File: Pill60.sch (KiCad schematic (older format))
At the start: 160 parts, among them J1 OLED, SW1 Rotary_Encoder_Switch, U1 ChinaBluePill

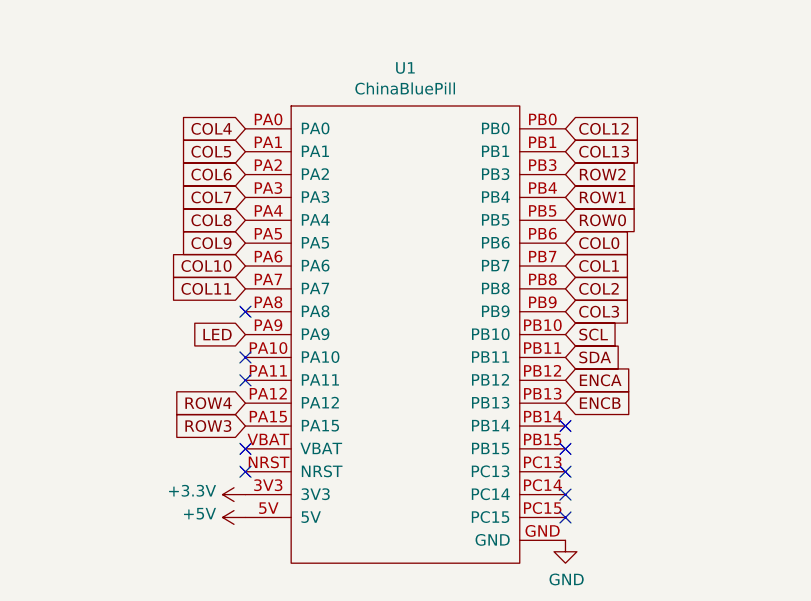
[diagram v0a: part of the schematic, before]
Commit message: Fix wires and make stuff better
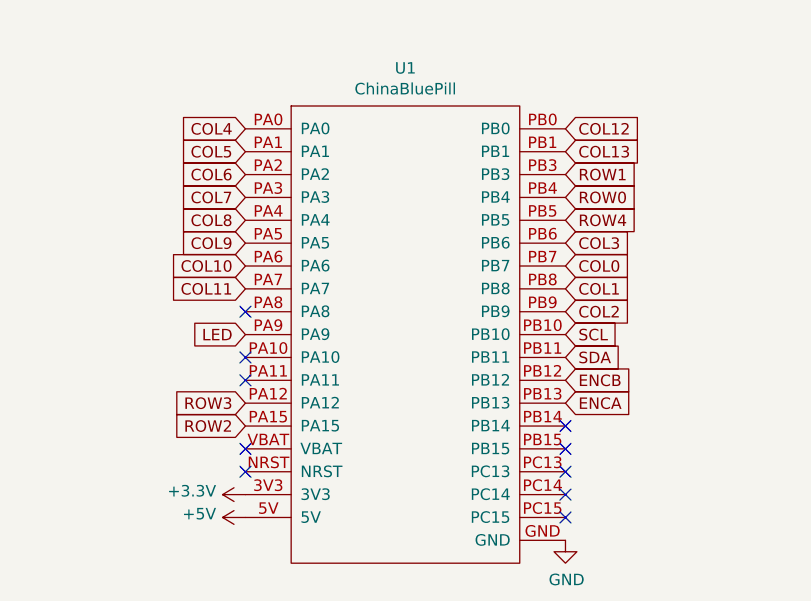
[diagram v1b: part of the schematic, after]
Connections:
- net COL0: now also U1.PB7; no longer U1.PB6
- net COL1: now also U1.PB8; no longer U1.PB7
- net COL2: now also U1.PB9; no longer U1.PB8
- net COL3: now also U1.PB6; no longer U1.PB9
- net ENCA: now also U1.PB13; no longer U1.PB12
- net ENCB: now also U1.PB12; no longer U1.PB13
- net ROW0: now also U1.PB4; no longer U1.PB5
- net ROW1: now also U1.PB3; no longer U1.PB4
- net ROW2: now also U1.PA15; no longer U1.PB3
- net ROW3: now also U1.PA12; no longer U1.PA15
- net ROW4: now also U1.PB5; no longer U1.PA12
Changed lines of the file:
@@
 Text GLabel 4950 1750 0    50   Input ~ 0
 ENCB
+Text GLabel 13100 3200 2    50   Input ~ 0
+ENCA
 Text GLabel 13100 3100 2    50   Input ~ 0
-ENCA
-Text GLabel 13100 3200 2    50   Input ~ 0
 ENCB
 $Comp
@@
 	0    -1   -1   0
 $EndComp
+Text GLabel 13100 2400 2    50   Input ~ 0
+ROW4
 Text GLabel 11700 3200 0    50   Input ~ 0
-ROW4
+ROW3
 Text GLabel 11700 3300 0    50   Input ~ 0
-ROW3
+ROW2
 Text GLabel 13100 2200 2    50   Input ~ 0
-ROW2
-Text GLabel 13100 2300 2    50   Input ~ 0
 ROW1
 $Comp
@@
 	1    0    0    -1
 $EndComp
+Text GLabel 13100 2500 2    50   Input ~ 0
+COL3
 Text GLabel 13100 2800 2    50   Input ~ 0
-COL3
+COL2
 Text GLabel 13100 2700 2    50   Input ~ 0
-COL2
-Text GLabel 13100 2600 2    50   Input ~ 0
 COL1
 Connection ~ 4200 5950
@@
 NoConn ~ 13100 3600
 NoConn ~ 13100 3700
-Text GLabel 13100 2500 2    50   Input ~ 0
+Text GLabel 13100 2600 2    50   Input ~ 0
 COL0
-Text GLabel 13100 2400 2    50   Input ~ 0
+Text GLabel 13100 2300 2    50   Input ~ 0
 ROW0
 Text GLabel 11700 2900 0    50   Input ~ 0
